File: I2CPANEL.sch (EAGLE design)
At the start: 47 parts, among them IC1 ATMEGA32U4-QFN

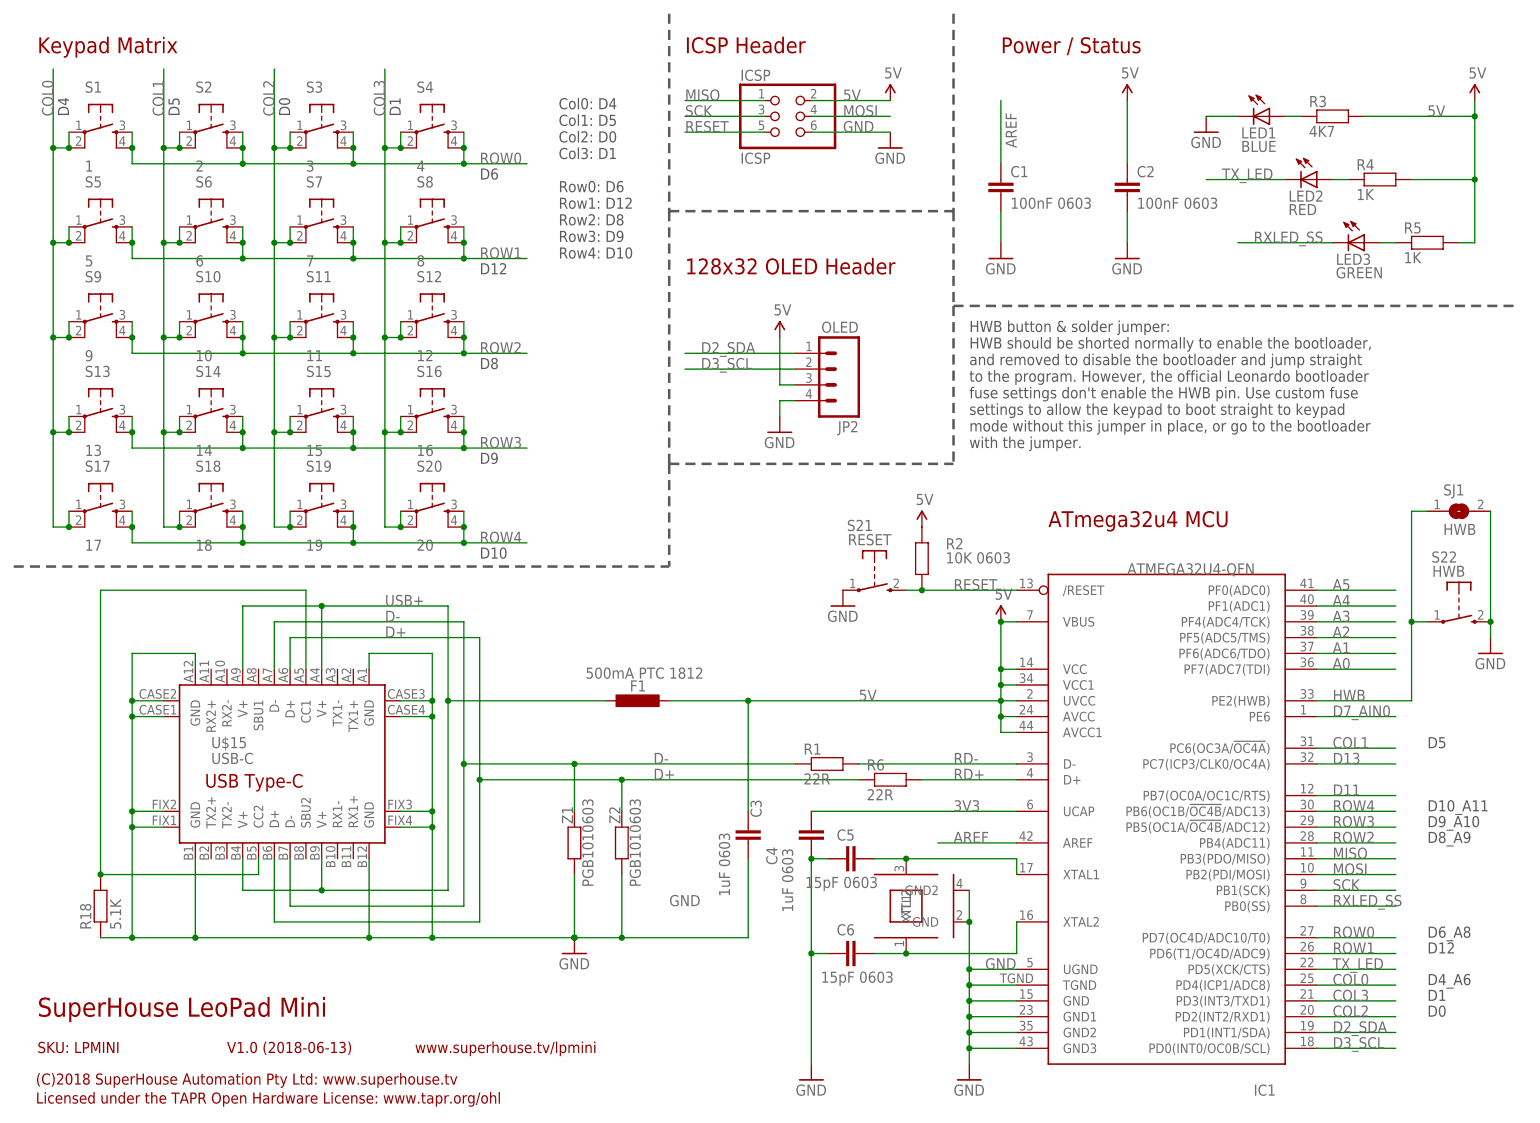
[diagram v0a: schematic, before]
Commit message: Schematic and routing for v1.0 release
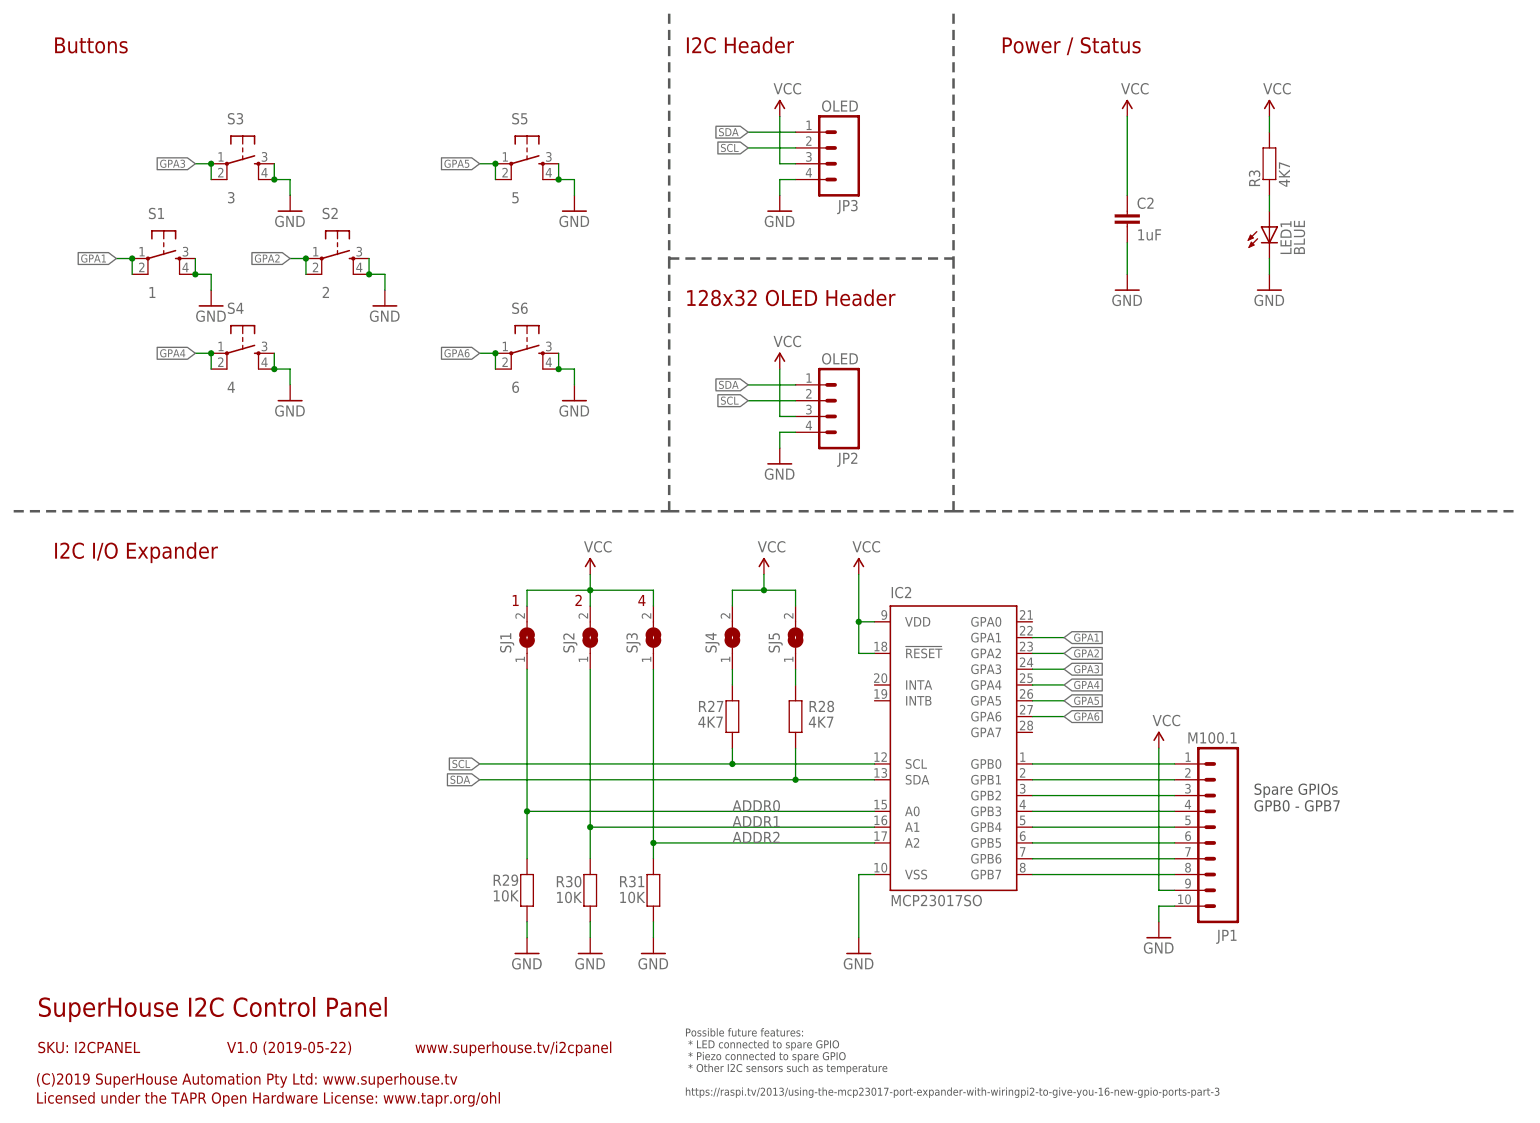
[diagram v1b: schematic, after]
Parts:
- removed C1: 100nF 0603, freetronics-master-v1.1:CAP0603
- removed C3, C4: 1uF 0603, freetronics-master-v1.1:CAP0603
- removed C5, C6: 15pF 0603, freetronics-master-v1.1:CAP0603
- removed F1: 500mA PTC 1812, rcl:L-EUL1812
- removed IC1: ATMEGA32U4-QFN, freetronics-jon:ATMEGA32U4-QFN
- removed ICSP: ICSP, pinhead:PINHD-2X3
- removed LED2: RED, freetronics-jon:LED0603
- removed LED3: GREEN, freetronics-jon:LED0603
- removed R1, R6: 22R, freetronics-jon:RESISTOR0603
- removed R18: 5.1K, freetronics-original:RESISTOR0603
- removed R2: 10K 0603, freetronics-master-v1.1:RESISTOR0603
- removed R4, R5: 1K, freetronics-jon:RESISTOR0603
- removed S10: 10, freetronics-original:TAC_SWITCHPTH
- removed S11: 11, freetronics-original:TAC_SWITCHPTH
- removed S12: 12, freetronics-original:TAC_SWITCHPTH
- removed S13: 13, freetronics-original:TAC_SWITCHPTH
- removed S14: 14, freetronics-original:TAC_SWITCHPTH
- removed S15: 15, freetronics-original:TAC_SWITCHPTH
- removed S16: 16, freetronics-original:TAC_SWITCHPTH
- removed S17: 17, freetronics-original:TAC_SWITCHPTH
- removed S18: 18, freetronics-original:TAC_SWITCHPTH
- removed S19: 19, freetronics-original:TAC_SWITCHPTH
- removed S20: 20, freetronics-original:TAC_SWITCHPTH
- removed S21: RESET, freetronics-jon:TAC_SWITCH_2PINSMT
- removed S22: HWB, freetronics-jon:TAC_SWITCH_2PINSMT
- removed S7: 7, freetronics-original:TAC_SWITCHPTH
- removed S8: 8, freetronics-original:TAC_SWITCHPTH
- removed S9: 9, freetronics-original:TAC_SWITCHPTH
- removed U$15: USB-C, freetronics-jon:USB-C
- removed XTL1: 16MHz, freetronics-jon:CRYSTAL-GND3X2
- removed Z1, Z2: PGB1010603, freetronics-master-v1.1:RESISTOR0603
- added IC2: MCP23017SO, microchip:MCP23017SO
- added JP1: M100.1, freetronics-original:M100.1
- added JP3: OLED, freetronics-jon:M04PTH
- added R27, R28: 4K7, freetronics-master-v1:RESISTOR0603
- added R29, R30, R31: 10K, freetronics-master-v1:RESISTOR0603
- added SJ2, SJ3, SJ4, SJ5: (no value), freetronics-jon:SJN
- C2: value 100nF 0603 -> 1uF
- SJ1: value HWB -> (none)
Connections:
- removed net 3V3: C4.2, IC1.UCAP
- removed net 5V: C2.1, C3.1, F1.2, IC1.AVCC, IC1.AVCC1, IC1.UVCC, IC1.VBUS, IC1.VCC, IC1.VCC1, ICSP.2, JP2.3, R2.2, R3.2, R4.2, R5.2
- removed net A0: IC1.PF7(ADC7(TDI)
- removed net A1: IC1.PF6(ADC6/TDO)
- removed net A2: IC1.PF5(ADC5/TMS)
- removed net A3: IC1.PF4(ADC4/TCK)
- removed net A4: IC1.PF1(ADC1)
- removed net A5: IC1.PF0(ADC0)
- removed net AREF: C1.1, IC1.AREF
- removed net COL0: IC1.PD4(ICP1/ADC8), S1.1, S1.2, S13.1, S13.2, S17.1, S17.2, S5.1, S5.2, S9.1, S9.2
- removed net COL1: IC1.PC6(OC3A/!OC4A!), S10.1, S10.2, S14.1, S14.2, S18.1, S18.2, S2.1, S2.2, S6.1, S6.2
- removed net COL2: IC1.PD2(INT2/RXD1), S11.1, S11.2, S15.1, S15.2, S19.1, S19.2, S3.1, S3.2, S7.1, S7.2
- removed net COL3: IC1.PD3(INT3/TXD1), S12.1, S12.2, S16.1, S16.2, S20.1, S20.2, S4.1, S4.2, S8.1, S8.2
- removed net D+: R6.1, U$15.D+@A6, U$15.D+@B6, Z2.2
- removed net D-: R1.1, U$15.D-@A7, U$15.D-@B7, Z1.2
- removed net D11: IC1.PB7(OC0A/OC1C/RTS)
- removed net D13: IC1.PC7(ICP3/CLK0/OC4A)
- removed net D2_SDA: IC1.PD1(INT1/SDA), JP2.1
- removed net D3_SCL: IC1.PD0(INT0/OC0B/SCL), JP2.2
- removed net D7_AIN0: IC1.PE6
- removed net HWB: IC1.PE2(HWB), S22.P, SJ1.1
- removed net MISO: IC1.PB3(PDO/MISO), ICSP.1
- removed net MOSI: IC1.PB2(PDI/MOSI), ICSP.4
- removed net N$11: C5.2, IC1.XTAL1, XTL1.XTL2
- removed net N$12: C6.2, IC1.XTAL2, XTL1.XTL1
- removed net N$67: R18.2, U$15.CC1, U$15.CC2
- removed net RD+: IC1.D+, R6.2
- removed net RD-: IC1.D-, R1.2
- removed net RESET: IC1./RESET, ICSP.5, R2.1, S21.S
- removed net ROW0: IC1.PD7(OC4D/ADC10/T0), S1.3, S1.4, S2.3, S2.4, S3.3, S3.4, S4.3, S4.4
- removed net ROW1: IC1.PD6(T1/OC4D/ADC9), S5.3, S5.4, S6.3, S6.4, S7.3, S7.4, S8.3, S8.4
- removed net ROW2: IC1.PB4(ADC11), S10.3, S10.4, S11.3, S11.4, S12.3, S12.4, S9.3, S9.4
- removed net ROW3: IC1.PB5(OC1A/!OC4B!/ADC12), S13.3, S13.4, S14.3, S14.4, S15.3, S15.4, S16.3, S16.4
- removed net ROW4: IC1.PB6(OC1B/!OC4B!/ADC13), S17.3, S17.4, S18.3, S18.4, S19.3, S19.4, S20.3, S20.4
- removed net RXLED_SS: IC1.PB0(SS), LED3.C
- removed net SCK: IC1.PB1(SCK), ICSP.3
- removed net TX_LED: IC1.PD5(XCK/CTS), LED2.C
- removed net USB+: F1.1, U$15.V+@A4, U$15.V+@A9, U$15.V+@B4, U$15.V+@B9
- new net ADDR0: IC2.A0, R29.2, SJ1.1
- new net ADDR1: IC2.A1, R30.2, SJ2.1
- new net ADDR2: IC2.A2, R31.2, SJ3.1
- new net GPA1: IC2.GPA1, S1.1, S1.2
- new net GPA2: IC2.GPA2, S2.1, S2.2
- new net GPA3: IC2.GPA3, S3.1, S3.2
- new net GPA4: IC2.GPA4, S4.1, S4.2
- new net GPA5: IC2.GPA5, S5.1, S5.2
- new net GPA6: IC2.GPA6, S6.1, S6.2
- new net N$1: IC2.GPB0, JP1.1
- new net N$2: IC2.GPB1, JP1.2
- new net N$3: IC2.GPB2, JP1.3
- new net N$4: IC2.GPB3, JP1.4
- new net N$42: R27.2, SJ4.1
- new net N$43: R28.2, SJ5.1
- new net N$5: IC2.GPB4, JP1.5
- new net N$9: IC2.GPB7, JP1.8
- new net SCL: IC2.SCL, JP2.2, JP3.2, R27.1
- new net SDA: IC2.SDA, JP2.1, JP3.1, R28.1
- new net VCC: C2.1, IC2.!RESET, IC2.VDD, JP1.9, JP2.3, JP3.3, R3.2, SJ1.2, SJ2.2, SJ3.2, SJ4.2, SJ5.2
- net GND: now also IC2.VSS, JP1.10, JP3.4, R29.1, R30.1, R31.1, S1.3, S1.4, S2.3, S2.4, S3.3, S3.4, S4.3, S4.4, S5.3, S5.4, S6.3, S6.4; no longer C1.2, C3.2, C4.1, C5.1, C6.1, IC1.GND, IC1.GND1, IC1.GND2, IC1.GND3, IC1.TGND, IC1.UGND, ICSP.6, R18.1, S21.P, S22.S, SJ1.2, U$15.GND@A1, U$15.GND@A12, U$15.GND@B1, U$15.GND@B12, U$15.GND@CASE1, U$15.GND@CASE2, U$15.GND@CASE3, U$15.GND@CASE4, U$15.GND@FIX1, U$15.GND@FIX2, U$15.GND@FIX3, U$15.GND@FIX4, XTL1.GND, XTL1.GND2, Z1.1, Z2.1
- net N$7: now also IC2.GPB5, JP1.6; no longer LED2.A, R4.1
- net N$8: now also IC2.GPB6, JP1.7; no longer LED3.A, R5.1
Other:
- note added: "(C)2019 SuperHouse Automation Pty Ltd: www.superhouse.tv"
- note added: "1"
- note added: "2"
- note added: "4"
- note added: "Buttons"
- note added: "I2C Header"
- note added: "I2C I/O Expander"
- note added: "Possible future features: * LED connected to spare GPIO * Piezo connected to spare GPIO * Other I2C sensors such as temperature https://raspi.tv/2013/using-the-mcp23017-port-expander-with-wiringpi2-to-give-you-16-new-gpio-ports-part-3"
- note added: "SKU: I2CPANEL"
- note added: "Spare GPIOs GPB0 - GPB7"
- note added: "SuperHouse I2C Control Panel"
- note added: "V1.0 (2019-05-22)"
- note added: "www.superhouse.tv/i2cpanel"
- note removed: "(C)2018 SuperHouse Automation Pty Ltd: www.superhouse.tv"
- note removed: "ATmega32u4 MCU"
- note removed: "Col0: D4 Col1: D5 Col2: D0 Col3: D1 Row0: D6 Row1: D12 Row2: D8 Row3: D9 Row4: D10"
- note removed: "D0"
- note removed: "D1"
- note removed: "D10"
- note removed: "D10_A11"
- note removed: "D12"
- note removed: "D4"
- note removed: "D4_A6"
- note removed: "D5"
- note removed: "D6"
- note removed: "D6_A8"
- note removed: "D8"
- note removed: "D8_A9"
- note removed: "D9"
- note removed: "D9_A10"
- note removed: "HWB button & solder jumper: HWB should be shorted normally to enable the bootloader, and removed to disable the bootloader and jump straight to the program. However, the official Leonardo bootloader fuse settings don't enable the HWB pin. Use custom fuse settings to allow the keypad to boot straight to keypad mode without this jumper in place, or go to the bootloader with the jumper."
- note removed: "ICSP Header"
- note removed: "Keypad Matrix"
- note removed: "SKU: LPMINI"
- note removed: "SuperHouse LeoPad Mini"
- note removed: "V1.0 (2018-06-13)"
- note removed: "www.superhouse.tv/lpmini"
- moved on the sheet: C2, JP2, LED1, R3, S1, S2, S3, S4, S5, S6, SJ1
